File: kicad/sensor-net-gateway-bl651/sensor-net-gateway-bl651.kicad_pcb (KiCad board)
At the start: 2 copper layers, 26 x 56 mm, 41 parts, among them M1 M50-3130545, M2 M50-3130545, SW1 PTS526_SM15_SMTR2_LFS, U1 USB_micro_ab, U2 USBLC6-2SC6, U3 FT230XQ, Y1 32.768 kHz

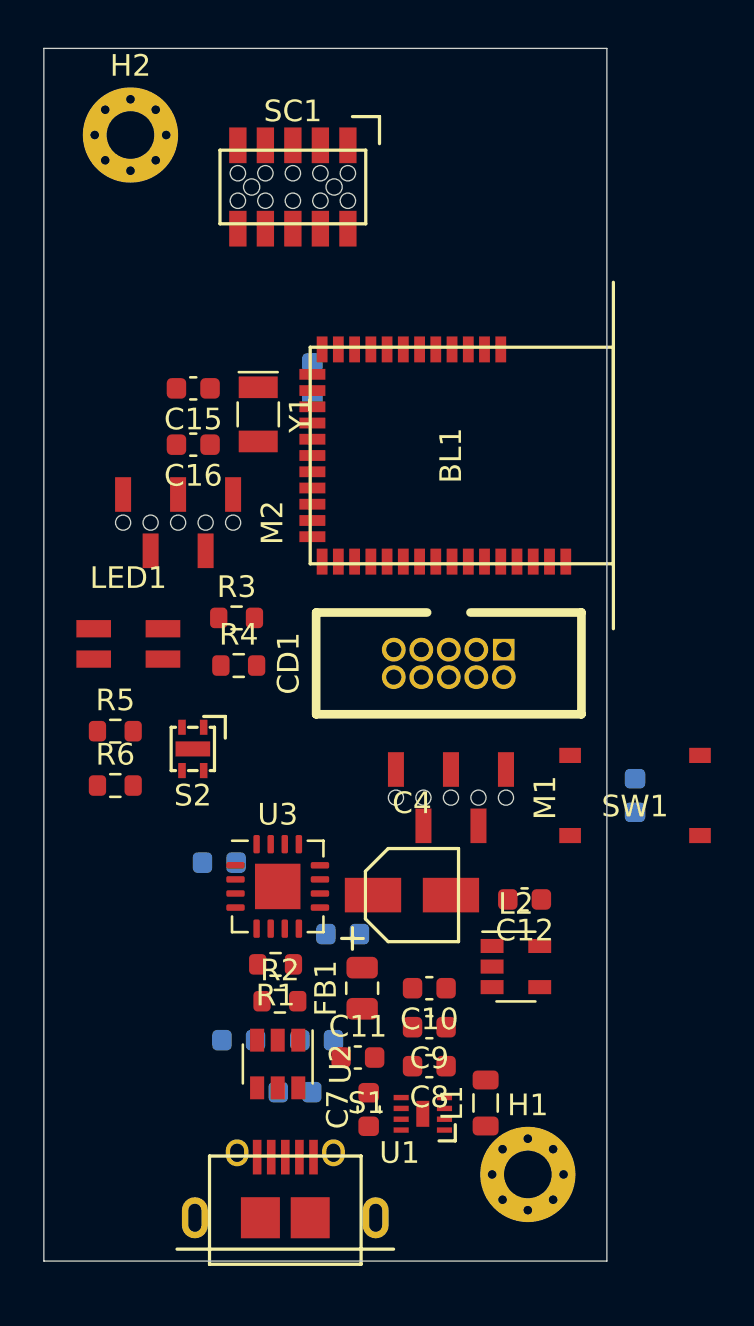
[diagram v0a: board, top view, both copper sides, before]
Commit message: routing snapshot
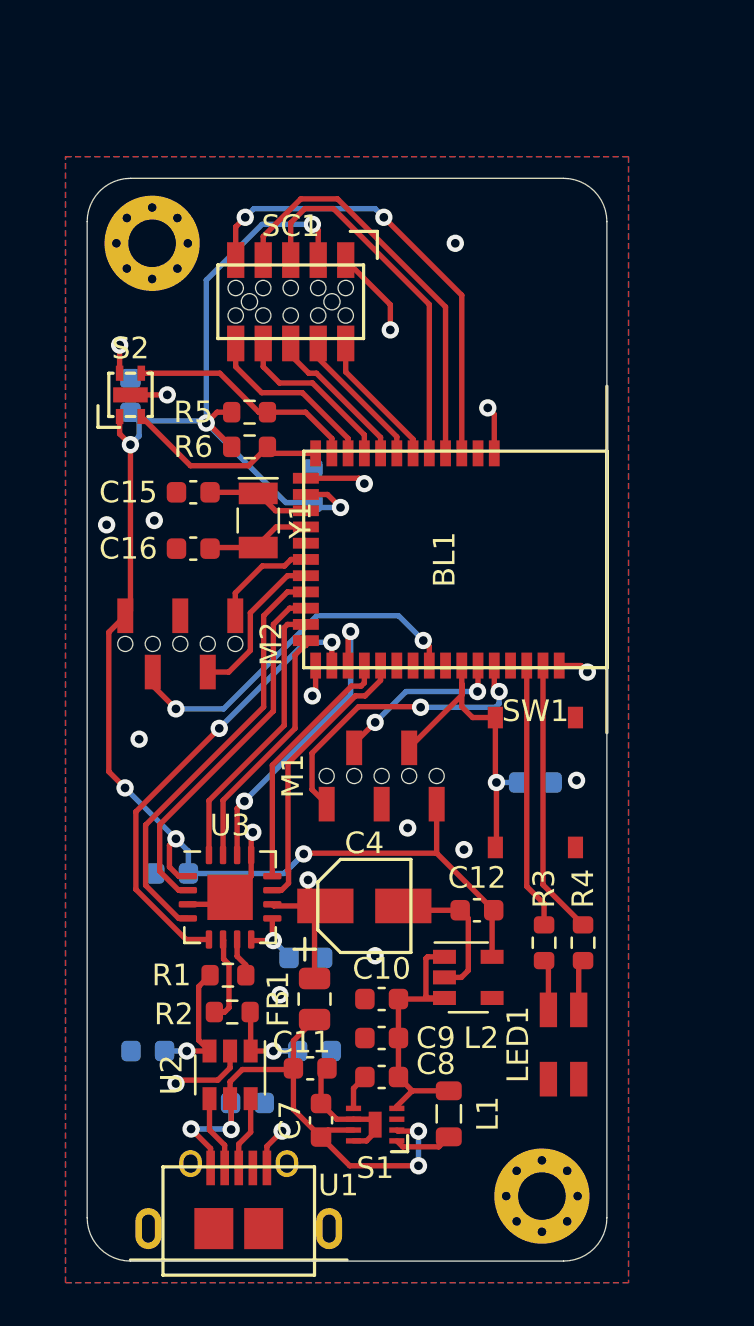
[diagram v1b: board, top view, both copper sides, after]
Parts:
- removed CD1: CORTEX-DEBUG, HH_CNCTech:CORTEX-DEBUG
- added C17: 0.1µF, Capacitor_SMD:C_0603_1608Metric, B.Cu at (154.0, 92.0)
- added L3: logo, HH_Hochreiner:logo, B.Cu at (168.0, 119.0)
- moved LED1 27.3 mm to (174.0, 122.0), turned to 90 degrees
- moved R3 20.7 mm to (173.1, 117.3), turned to 270 degrees
- moved R4 20.4 mm to (174.9, 117.3), turned to 270 degrees
- moved R6 16.8 mm to (159.5, 94.4)
- moved S2 16.6 mm to (154.0, 92.0), turned to 180 degrees
- moved R5 16.0 mm to (159.5, 92.8)
- moved M2 5.60 mm to (156.3, 103.5)
- moved SC1 5.30 mm to (161.4, 87.7)
- moved H2 5.10 mm to (155.0, 85.0)
- moved C14 4.90 mm to (162.4, 96.2)
- moved Y1 4.90 mm to (159.9, 97.8)
- moved BL1 4.81 mm to (169.0, 99.6)
- moved C15 4.80 mm to (156.9, 96.5)
- moved C16 4.80 mm to (156.9, 99.1)
- moved C13 4.64 mm to (172.7, 109.9), turned to 0 degrees
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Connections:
- net Net-(U1-Pad2) renamed /usb/D_N
- net Net-(U1-Pad3) renamed /usb/D_P
- BL1 pad 12: /mcu/FTDI_DIO0 -> /mcu/FTDI_DIO1
- BL1 pad 13: /mcu/FTDI_DIO1 -> /mcu/FTDI_DIO0
- BL1 pad 14: /mcu/FTDI_DIO2 -> /mcu/FTDI_DIO3
- BL1 pad 15: /mcu/FTDI_DIO3 -> /mcu/FTDI_DIO2
- BL1 pad 2: /mcu/SPI_MISO -> /mcu/LED_GREEN
- BL1 pad 21: (no net) -> /mcu/UART2.TX
- BL1 pad 22: (no net) -> /mcu/UART2.RX
- BL1 pad 28: (no net) -> /sensor/SCL
- BL1 pad 3: /mcu/SPI_MOSI -> /mcu/LED_RED
- BL1 pad 30: /sensor/SCL -> /mcu/GPIO_2
- BL1 pad 31: /mcu/LED_GREEN -> /mcu/~SPI_CS
- BL1 pad 32: /mcu/LED_RED -> /mcu/SPI_CLK
- BL1 pad 33: /mcu/GPIO_2 -> /mcu/SPI_MOSI
- BL1 pad 34: /mcu/GPIO_1 -> /mcu/SPI_MISO
- BL1 pad 35: /mcu/~SPI_CS -> /mcu/I2C_SDA
- BL1 pad 37: /mcu/I2C_SDA -> /mcu/GPIO_1
- BL1 pad 38: /mcu/SPI_CLK -> (no net)
- C1 pad 2: /power/GND -> GND
- C10 pad 2: /power/GND -> GND
- C11 pad 2: /power/GND -> GND
- C12 pad 2: /power/GND -> GND
- C2 pad 2: /power/GND -> GND
- C21 pad 2: /power/GND -> GND
- C3 pad 2: /power/GND -> GND
- C4 pad 2: /power/GND -> GND
- C5 pad 2: /power/GND -> GND
- C6 pad 1: /power/GND -> GND
- C7 pad 2: /power/GND -> GND
- C9 pad 2: /power/GND -> GND
- L2 pad 2: /power/GND -> GND
- M2 pad 1: /usb/UART.RX -> /power/3V0
- M2 pad 2: /usb/UART.TX -> /mcu/SWO
- M2 pad 4: /usb/UART.RTS -> /mcu/UART2.TX
- M2 pad 5: /usb/UART.CTS -> /mcu/UART2.RX
- S1 pad 6: /power/GND -> GND
- S1 pad 8: /power/GND -> GND
- S2 pad 4: /power/GND -> GND
- U1 pad 5: /power/GND -> GND
- U2 pad 2: /power/GND -> GND
- U3 pad 13: /power/GND -> GND
- U3 pad 17: /power/GND -> GND
- U3 pad 3: /power/GND -> GND
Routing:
- net /power/3V0: track 0.00 -> 77.7 mm, vias 0 -> 7
- net GND: track 0.00 -> 39.1 mm, vias 0 -> 19
- net /power/VBUS: track 0.00 -> 26.3 mm, vias 0 -> 4
- net /mcu/FTDI_DIO2: track 0.00 -> 21.3 mm, vias 0 -> 2
- net /mcu/GPIO_1: track 0.00 -> 21.3 mm, vias 0 -> 2
- net /usb/UART.CTS: track 0.00 -> 19.7 mm
- net /mcu/I2C_SCL: track 0.00 -> 19.1 mm
- net /mcu/I2C_SDA: track 0.00 -> 17.1 mm
- net /mcu/SWO: track 0.00 -> 17.1 mm, vias 0 -> 2
- net /usb/UART.RX: track 0.00 -> 17.0 mm
- net /mcu/~RESET: track 0.00 -> 14.7 mm, vias 0 -> 1
- net /mcu/FTDI_DIO3: track 0.00 -> 14.1 mm, vias 0 -> 2
- net /mcu/SWDIO: track 0.00 -> 14.1 mm, vias 0 -> 2
- net /usb/UART.RTS: track 0.00 -> 13.0 mm
- net /mcu/FTDI_DIO1: track 0.00 -> 13.0 mm
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- added copper zone on B.Cu, net GND
- added copper zone on F.Cu, net GND
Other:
- board size 26 x 56 mm -> 24 x 50 mm
